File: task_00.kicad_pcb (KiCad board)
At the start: 2 copper layers, 36.6 x 31.3 mm, 36 parts, among them J1 Screw_Terminal_01x02, 3935700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, J2 Screw_Terminal_01x02, 3935700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, Q1 FQP27P06, U1 TPS54360DDAR

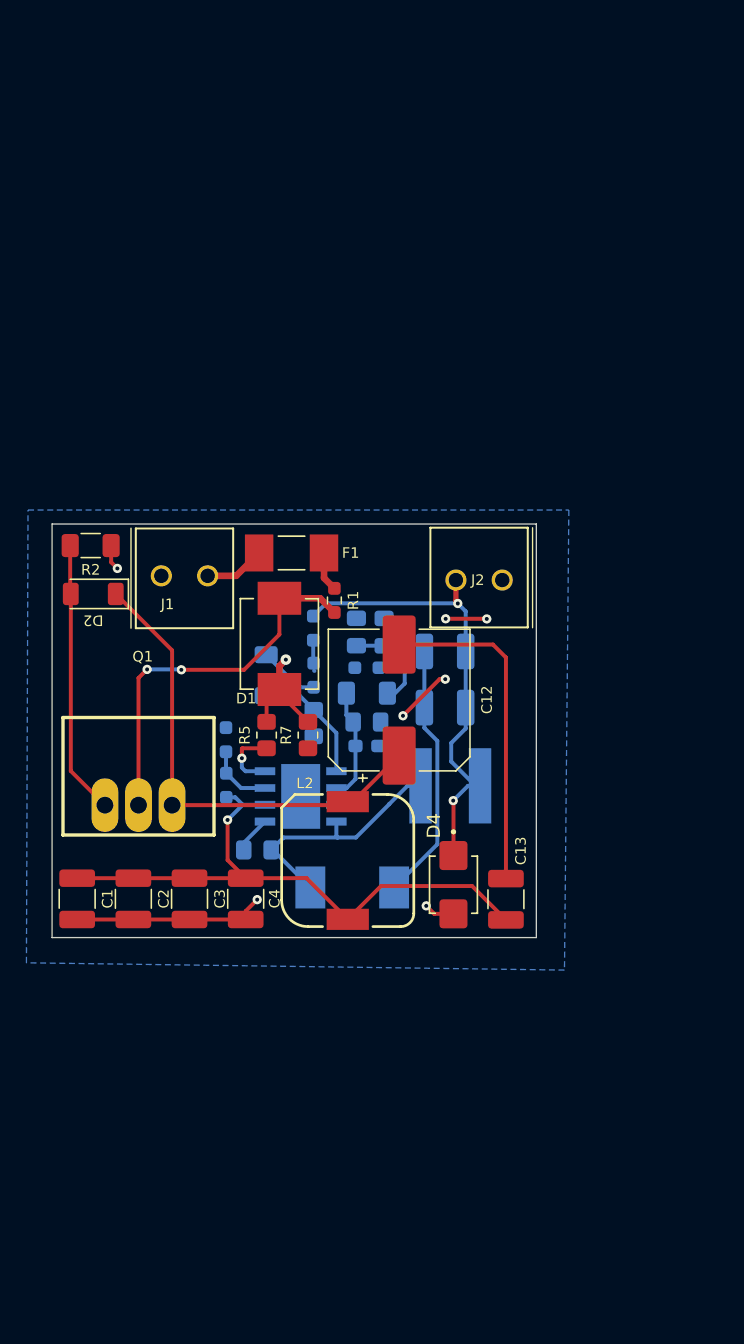
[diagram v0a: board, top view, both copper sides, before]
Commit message: version 2
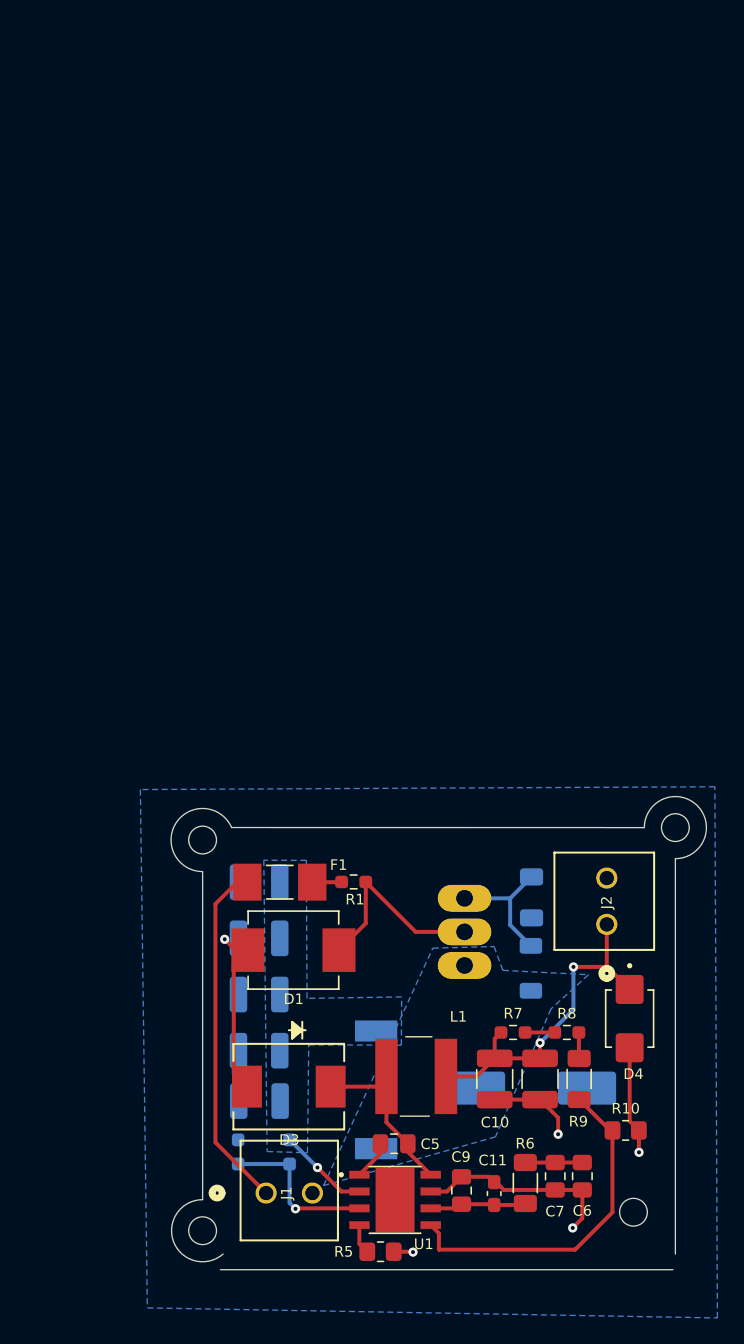
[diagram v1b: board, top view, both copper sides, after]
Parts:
- removed the R4 at (104.2, 93.4)
- removed the R4 at (114.8, 87.9)
- removed the R7 at (110.4, 93.0)
- removed the R7 at (110.8, 84.9)
- added H1: MountingHole, MountingHole:MountingHole_2.1mm, F.Cu at (135.0, 129.1)
- added H2: MountingHole, MountingHole:MountingHole_2.1mm, F.Cu at (102.4, 101.0)
- added H3: MountingHole, MountingHole:MountingHole_2.1mm, F.Cu at (102.4, 130.5)
- added H4: MountingHole, MountingHole:MountingHole_2.1mm, F.Cu at (138.2, 100.0)
- added R4: 84.5k, 0603WAF8452T5E, Resistor_SMD:R_0603_1608Metric_Pad0.98x0.95mm_HandSolder, B.Cu at (105.1, 124.5)
- added R7: 30k, RC0603JR-0730KL, Resistor_SMD:R_0603_1608Metric_Pad0.98x0.95mm_HandSolder, F.Cu at (125.9, 115.5)
- C1, C12, C13, C2, C3, C4, D2, L2, Q1, R2: moved to B.Cu
- C10, C11, C5, C6, C7, C8, C9, D3, L1, R10, R6, R8, R9, U1: moved to F.Cu
- moved J1 47.1 mm to (107.2, 127.7), turned to 0 degrees
- moved C7 43.8 mm to (129.1, 126.4), turned to -90 degrees
- moved C6 43.8 mm to (131.1, 126.4), turned to -90 degrees
- moved D2 43.5 mm to (127.2, 112.4), turned to 90 degrees
- moved R2 42.7 mm to (127.3, 105.3), turned to 90 degrees
- moved R5 40.0 mm to (115.9, 132.1), turned to 0 degrees
- moved R6 39.0 mm to (126.8, 126.9), turned to 90 degrees
- moved R10 38.8 mm to (134.4, 122.9), turned to 0 degrees
- moved R9 38.7 mm to (130.9, 119.0)
- moved C9 36.2 mm to (122.0, 127.5), turned to 90 degrees
- moved C11 35.2 mm to (124.5, 127.7), turned to 90 degrees
- moved C8 33.1 mm to (127.9, 119.0), turned to -90 degrees
- moved R8 33.1 mm to (130.0, 115.5), turned to 0 degrees
- moved U1 31.4 mm to (117.0, 128.2)
- moved C12 31.0 mm to (127.3, 119.7), turned to 0 degrees
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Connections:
- C10 pad 2: Net-(D3-A) -> GND
- C12 pad 2: Net-(C12-Pad2) -> GND
- C13 pad 2: Net-(C12-Pad2) -> GND
- C8 pad 2: Net-(D3-A) -> GND
- D3 pad 2: Net-(D3-A) -> GND
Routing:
- net /VIN: track 45.6 -> 6.90 mm
- net /VIN_sp: track 36.5 -> 0.00 mm
- net Net-(C12-Pad2): track 25.2 -> 0.00 mm
- net Net-(J1-Pin_1): track 4.61 -> 26.6 mm
- net Net-(D3-A): track 19.6 -> 0.00 mm
- net /FB: track 9.48 -> 26.1 mm
- net Net-(D1-Pad1): track 29.0 -> 15.0 mm, vias 2 -> 0
- net Net-(D2-A): track 20.7 -> 9.99 mm
- net /V_OUT: track 35.1 -> 26.0 mm
- net GND: track 37.8 -> 45.1 mm, vias 8 -> 5
- net /EN: track 5.04 -> 12.3 mm, vias 0 -> 1
- net Net-(D3-K): track 18.7 -> 13.4 mm
- net Net-(C6-Pad1): track 7.34 -> 4.31 mm
- net Net-(U1-RT/CLK): track 5.17 -> 2.26 mm, vias 1 -> 0
- net Net-(R8-Pad2): track 4.61 -> 1.98 mm
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- added copper zone on B.Cu, net /VIN
- added copper zone on B.Cu, net /VIN_sp
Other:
- board size 36.6 x 31.3 mm -> 40.5 x 35.8 mm

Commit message: Version 3
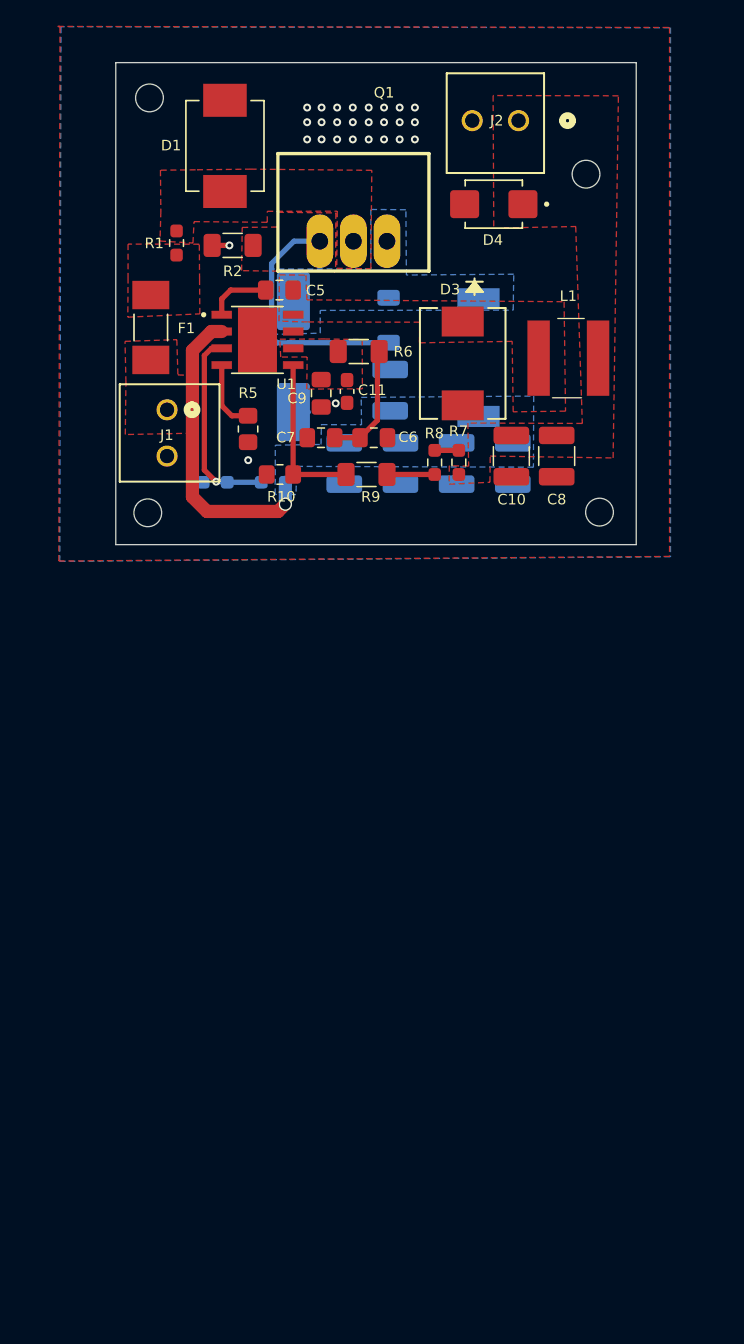
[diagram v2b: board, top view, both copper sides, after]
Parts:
- Q1, R2: moved to F.Cu
- moved H1 91.9 mm to (98.4, 44.8)
- moved H3 85.0 mm to (131.4, 50.6)
- moved U1 65.9 mm to (106.6, 63.1)
- moved C5 65.2 mm to (108.2, 59.3)
- moved R6 64.2 mm to (114.2, 64.0), turned to 0 degrees
- moved Q1 63.8 mm to (113.8, 44.2), turned to 0 degrees
- moved R5 63.1 mm to (105.8, 69.8), turned to -90 degrees
- moved D4 62.5 mm to (124.4, 52.8), turned to 180 degrees
- moved C11 61.7 mm to (113.3, 67.0), turned to -90 degrees
- moved C9 61.2 mm to (111.4, 67.2), turned to -90 degrees
- moved J2 61.2 mm to (126.3, 46.5), turned to 180 degrees
- moved D1 61.1 mm to (104.1, 48.4), turned to 90 degrees
- moved J1 59.7 mm to (99.7, 68.4), turned to -90 degrees
- moved C7 58.6 mm to (111.4, 70.5), turned to 180 degrees
- moved C12 58.2 mm to (109.3, 64.4), turned to -90 degrees
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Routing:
- net GND: track 45.1 -> 2.45 mm, vias 5 -> 27
- net Net-(J1-Pin_1): track 26.6 -> 0.00 mm
- net /V_OUT: track 26.0 -> 0.00 mm, vias 2 -> 0
- net /VIN: track 6.90 -> 23.3 mm
- net Net-(D1-Pad1): track 15.0 -> 0.00 mm
- net /FB: track 26.1 -> 12.3 mm
- net Net-(D3-K): track 13.4 -> 0.00 mm
- net Net-(D2-A): track 9.99 -> 19.0 mm
- net Net-(U1-COMP): track 7.36 -> 0.00 mm
- net Net-(C6-Pad1): track 4.31 -> 9.29 mm
- net Net-(U1-RT/CLK): track 2.26 -> 5.38 mm
- net /EN: track 12.3 -> 14.9 mm
- net Net-(F1-Pad2): track 2.23 -> 0.00 mm
- net Net-(U1-BOOT): track 3.00 -> 4.80 mm
- net Net-(R8-Pad2): track 1.98 -> 3.61 mm
- added copper zone on F.Cu, net /V_OUT
- added copper zone on F.Cu, net GND
- added copper zone on F.Cu, net Net-(D1-Pad1)
- added copper zone on F.Cu, net Net-(D2-A)
- added copper zone on F.Cu, net Net-(D3-K)
- added copper zone on F.Cu, net Net-(F1-Pad2)
- added copper zone on F.Cu, net Net-(J1-Pin_1)
- added copper zone on F.Cu, net Net-(U1-COMP)
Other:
- board size 40.5 x 35.8 mm -> 39.4 x 36.5 mm
